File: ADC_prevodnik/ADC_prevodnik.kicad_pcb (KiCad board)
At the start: 2 copper layers, 9 parts, among them J1 Conn_01x10_Pin, J2 Conn_01x04_Pin, J3 Conn_01x02_Pin

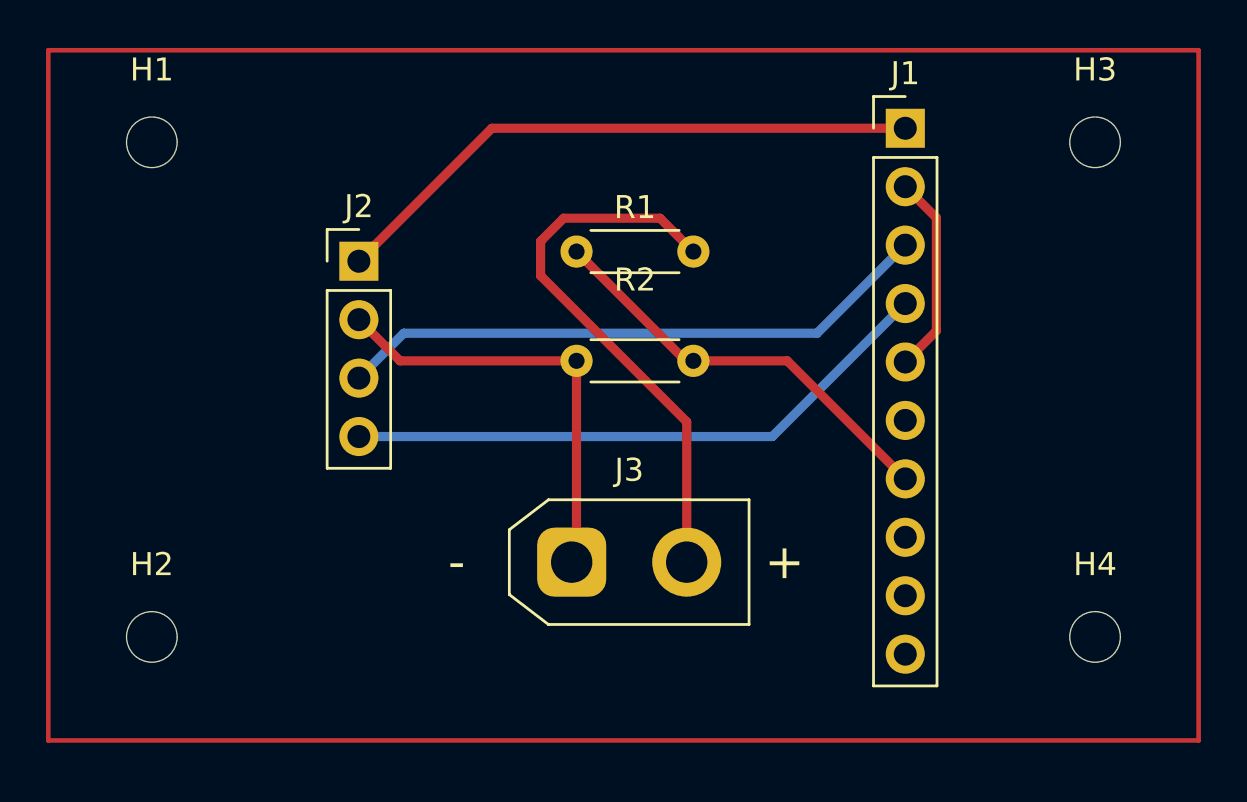
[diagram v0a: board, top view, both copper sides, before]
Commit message: 210426
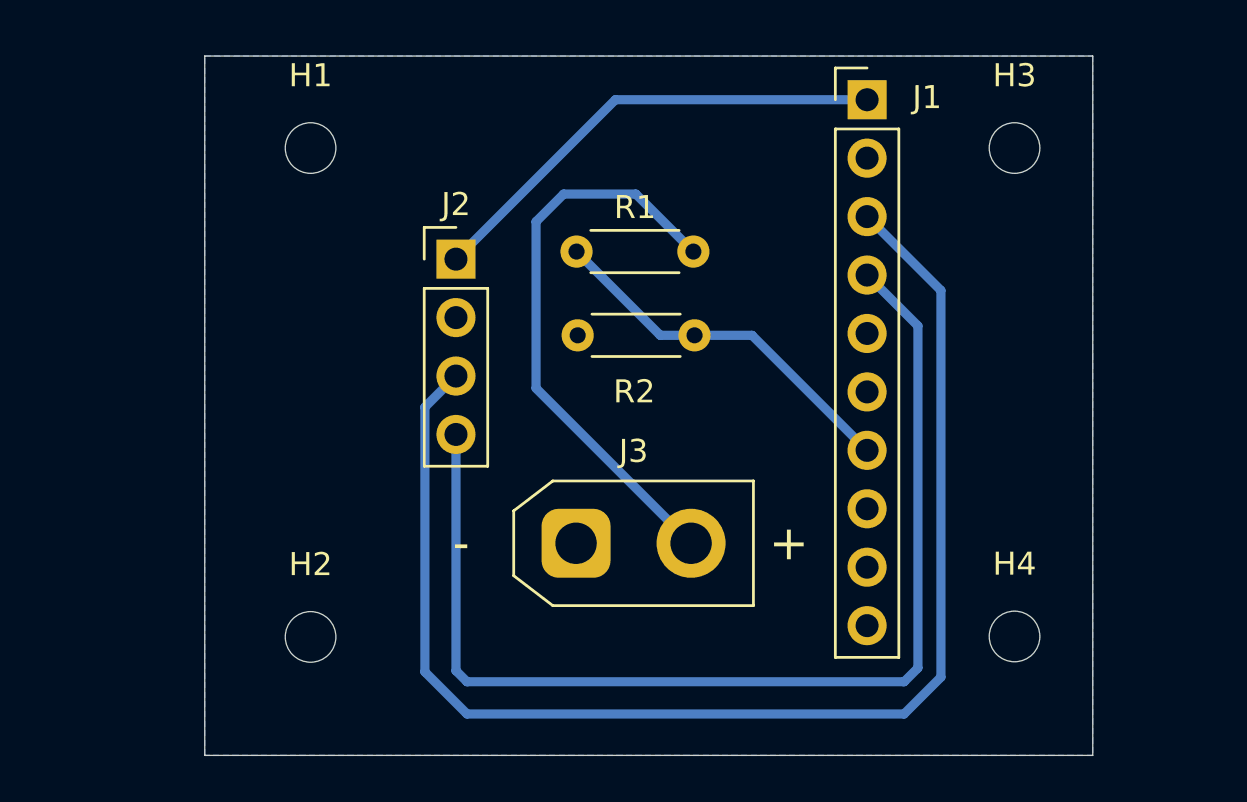
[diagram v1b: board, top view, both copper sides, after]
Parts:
- moved H1 6.90 mm to (138.4, 78.0)
- moved H2 6.90 mm to (138.4, 99.2)
- moved J2 4.22 mm to (144.7, 82.8)
- moved H3 3.51 mm to (169.0, 78.0)
- moved H4 3.50 mm to (169.0, 99.2)
- moved J1 2.07 mm to (162.6, 75.9)
- moved R2 1.11 mm to (150.0, 86.1)
- moved J3 0.84 mm to (149.9, 95.2)
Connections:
- net /ADDR renamed /GND
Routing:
- net /GPIO 21: track 26.1 -> 58.6 mm
- net /GND: track 27.8 -> 0.30 mm
- net /GPIO 22: track 26.1 -> 48.8 mm
- net /3,3V: track 26.1 -> 20.7 mm
- net /A0: track 18.4 -> 16.2 mm
- net /VCC: track 24.2 -> 25.1 mm
- added copper zone on B.Cu, net /GND
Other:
- board outline added: 38.6 x 30.4 mm
